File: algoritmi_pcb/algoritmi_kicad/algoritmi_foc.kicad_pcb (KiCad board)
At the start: 2 copper layers, 45.2 x 29.2 mm, 23 parts, among them J1 SSM-107-L-DV-P-TR, J2 53261-0371, J3 SSM-105-L-SH, U1 TMC6300-LA-T

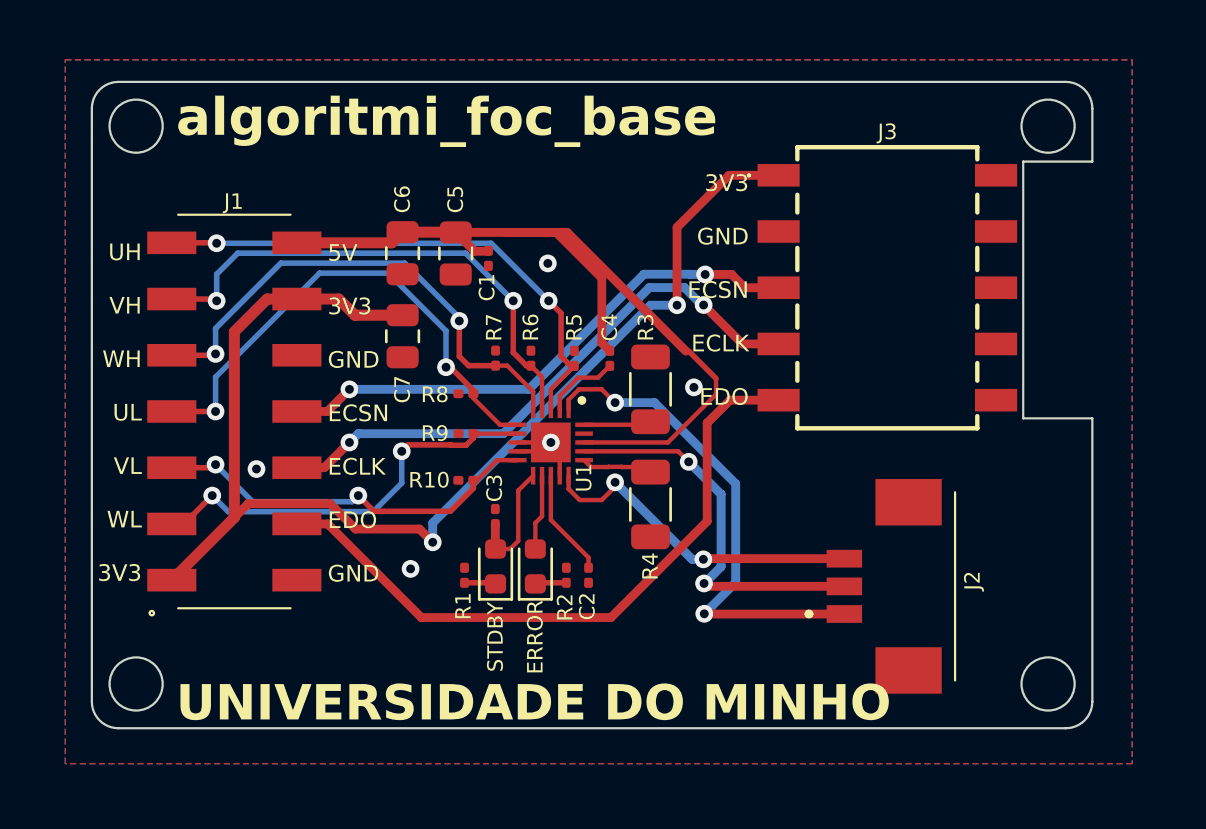
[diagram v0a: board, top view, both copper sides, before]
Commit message: Updated Gerbers Base PCB
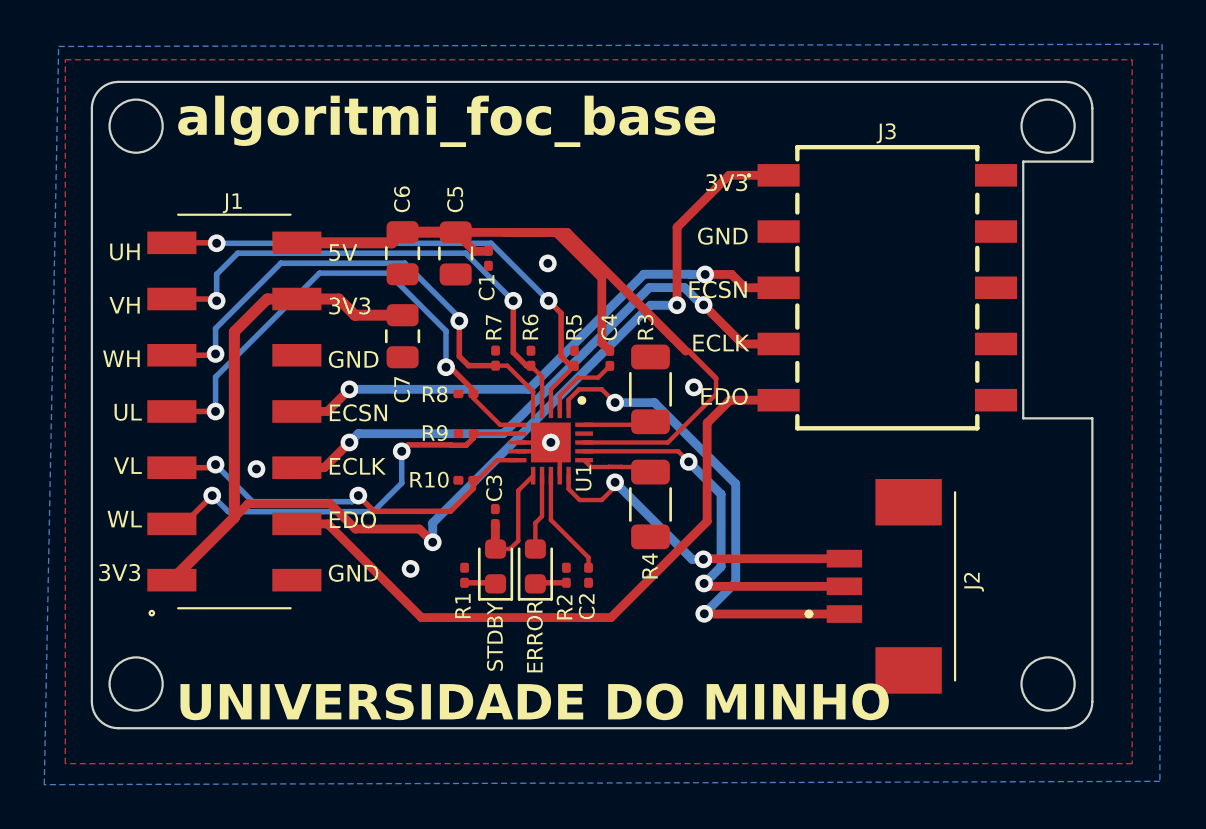
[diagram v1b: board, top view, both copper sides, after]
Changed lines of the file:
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@@
 			(drillshape 0)
 			(scaleselection 1)
-			(outputdirectory "algoritmi_foc_gerber/algoritmi_foc_map/")
+			(outputdirectory "algoritmi_foc_gerber/")
 		)
 	)
@@
 	)
 	(zone
-		(net 0)
-		(net_name "")
+		(net 1)
+		(net_name "GND")
 		(layer "F.Cu")
-		(name "a")
 		(hatch edge 0.5)
 		(connect_pads
@@
 		(min_thickness 0.25)
 		(filled_areas_thickness no)
-		(keepout
-			(tracks allowed)
-			(vias allowed)
-			(pads allowed)
-			(copperpour not_allowed)
-			(footprints allowed)
-		)
-		(fill
+		(fill yes
 			(thermal_gap 0.5)
 			(thermal_bridge_width 0.5)
@@
 		(polygon
 			(pts
-				(xy 84.4 85) (xy 84.4 86.4) (xy 84.6 86.4) (xy 85.2 85.8) (xy 85.2 85.4) (xy 85.4 85.2) (xy 85.8 85.2)
-				(xy 85.8 84.8) (xy 85.6 84.6) (xy 85 84.6) (xy 85 85)
+				(xy 79 66) (xy 127.2 66) (xy 127.2 97.8) (xy 79 97.8)
 			)
 		)
 	)
 	(zone
-		(net 1)
-		(net_name "GND")
-		(layers "F&B.Cu")
+		(net 0)
+		(net_name "")
+		(layer "F.Cu")
+		(name "a")
 		(hatch edge 0.5)
 		(connect_pads
@@
 		(min_thickness 0.25)
 		(filled_areas_thickness no)
-		(fill yes
+		(keepout
+			(tracks allowed)
+			(vias allowed)
+			(pads allowed)
+			(copperpour not_allowed)
+			(footprints allowed)
+		)
+		(fill
 			(thermal_gap 0.5)
 			(thermal_bridge_width 0.5)
@@
 		(polygon
 			(pts
-				(xy 79 66) (xy 127.2 66) (xy 127.2 97.8) (xy 79 97.8)
+				(xy 84.4 85) (xy 84.4 86.4) (xy 84.6 86.4) (xy 85.2 85.8) (xy 85.2 85.4) (xy 85.4 85.2) (xy 85.8 85.2)
+				(xy 85.8 84.8) (xy 85.6 84.6) (xy 85 84.6) (xy 85 85)
 			)
 		)
@@
 			)
 		)
+	)
+	(zone
+		(net 1)
+		(net_name "GND")
+		(layer "B.Cu")
+		(hatch edge 0.5)
+		(priority 1)
+		(connect_pads
+			(clearance 0)
+		)
+		(min_thickness 0.25)
+		(filled_areas_thickness no)
+		(fill yes
+			(thermal_gap 0.5)
+			(thermal_bridge_width 0.5)
+		)
+		(polygon
+			(pts
+				(xy 78.7 65.4) (xy 128.55 65.3) (xy 128.45 98.6) (xy 78.05 98.75)
+			)
+		)
